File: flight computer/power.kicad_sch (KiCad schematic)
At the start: 27 parts, among them J10 Conn_01x02_Pin, Q2 DMG2301L, U13 LTC4412xS6, U14 TPS61092, U15 AP2112K-3.3, U9 TPS82130

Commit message: daily commit
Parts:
- J10: footprint Connector_JST:JST_PH_B2B-PH-K_1x02_P2.00mm_Vertical -> TerminalBlock_Phoenix:TerminalBlock_Phoenix_MPT-0,5-2-2.54_1x02_P2.54mm_Horizontal
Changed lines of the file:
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@@
 			)
 		)
-		(property "Footprint" "Connector_JST:JST_PH_B2B-PH-K_1x02_P2.00mm_Vertical"
+		(property "Footprint" "TerminalBlock_Phoenix:TerminalBlock_Phoenix_MPT-0,5-2-2.54_1x02_P2.54mm_Horizontal"
 			(at 26.67 39.37 0)
 			(effects

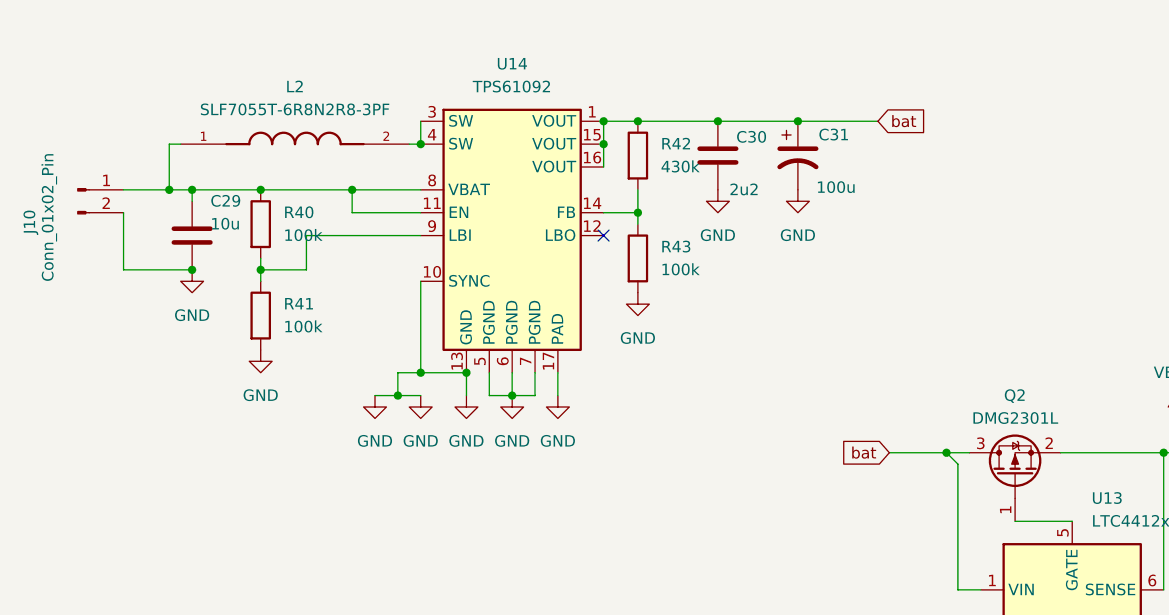
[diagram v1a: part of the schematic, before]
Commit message: power fixes
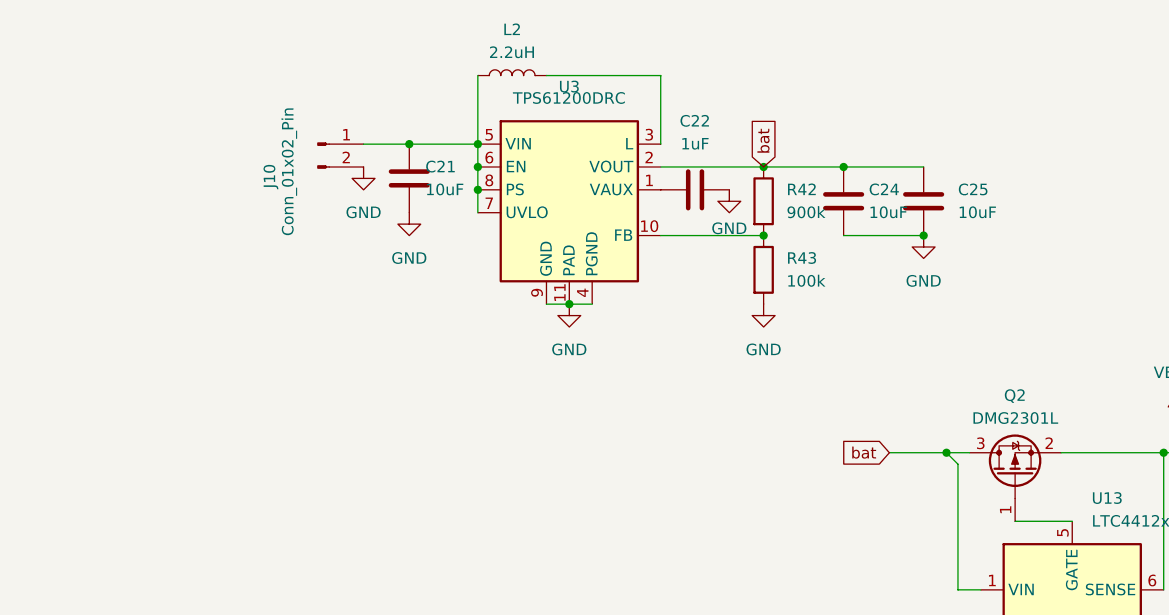
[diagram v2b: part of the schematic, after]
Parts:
- removed C29: 10u, Capacitor_SMD:C_0603_1608Metric, symbol Device:C
- removed C30: 2u2, Capacitor_SMD:C_0603_1608Metric, symbol Device:C
- removed C31: 100u, Capacitor_SMD:C_0603_1608Metric, symbol Device:C_Polarized_US
- removed L2: SLF7055T-6R8N2R8-3PF, Inductor_SMD:L_7.3x7.3_H4.5, symbol SLF7055T-6R8N2R8-3PF[1]:SLF7055T-6R8N2R8-3PF
- removed R40, R41: 100k, Resistor_SMD:R_0603_1608Metric, symbol Device:R
- removed U14: TPS61092, Package_DFN_QFN:Texas_RSA_VQFN-16-1EP_4x4mm_P0.65mm_EP2.7x2.7mm_ThermalVias, symbol Regulator_Switching:TPS61092
- added C21, C24, C25: 10uF, Capacitor_SMD:C_0603_1608Metric, symbol Device:C
- added C22: 1uF, Capacitor_SMD:C_0603_1608Metric, symbol Device:C
- added L2: 2.2uH, Inductor_SMD:L_APV_ANR4018, symbol Device:L
- added U3: TPS61200DRC, Package_SON:Texas_S-PVSON-N10_ThermalVias, symbol Regulator_Switching:TPS61200DRC
- R42: value 430k -> 900k
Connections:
- net GND: now also C21.2, C22.2, C24.2, C25.2, U3.11 (PAD), U3.4 (PGND), U3.9 (GND)
- net bat: now also C24.1, C25.1, U3.2 (VOUT)
- net at J10.1 (Pin_1): now also C21.1, L2.1, U3.5 (VIN), U3.6 (EN), U3.7 (UVLO), U3.8 (PS)
- net at R42.2, R43.1: now also U3.10 (FB)
- new net: C22.1, U3.1 (VAUX)
- new net: L2.2, U3.3 (L)
- no-connect marks 3 -> 2
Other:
- moved on the sheet: J10, R42, R43
